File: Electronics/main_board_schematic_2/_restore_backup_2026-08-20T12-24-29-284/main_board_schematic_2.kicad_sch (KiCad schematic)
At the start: 6 parts, among them J1 Conn_01x02_Pin, J2 Conn_01x02_Socket, U1 DEVKIT_V1_ESP32-WROOM-32, U2 L7805

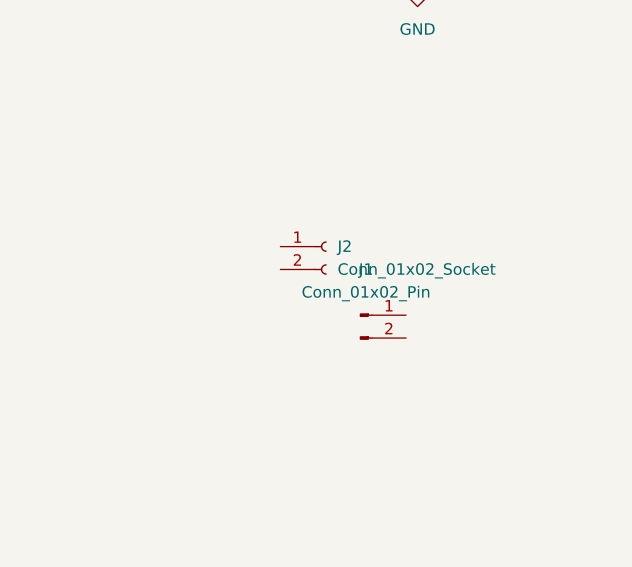
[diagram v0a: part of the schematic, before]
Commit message: start kicad version of board
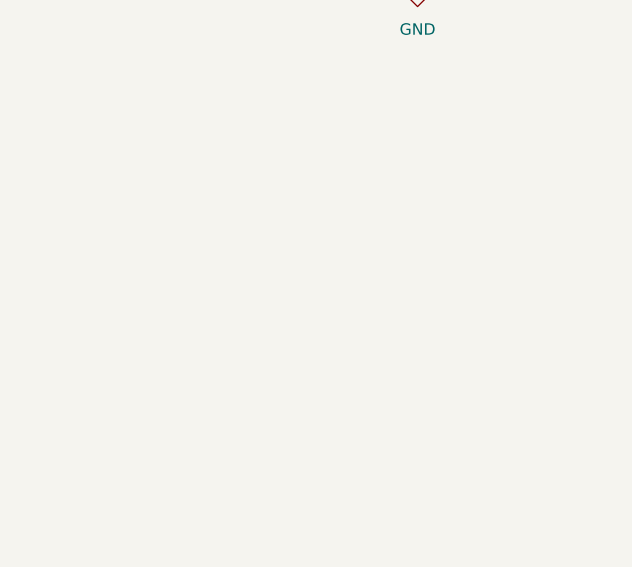
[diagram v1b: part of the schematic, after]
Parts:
- removed J1: Conn_01x02_Pin, Connector_JST:JST_XH_B2B-XH-AM_1x02_P2.50mm_Vertical, symbol Connector:Conn_01x02_Pin
- removed J2: Conn_01x02_Socket, Connector_JST:JST_XH_B2B-XH-A_1x02_P2.50mm_Vertical, symbol Connector:Conn_01x02_Socket
- U2: footprint Package_TO_SOT_THT:TO-220F-3_Horizontal_TabDown -> (none)
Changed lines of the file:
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@@
-	)
-	(symbol
-		(lib_id "Connector:Conn_01x02_Socket")
-		(at 203.2 82.55 0)
-		(unit 1)
-		(body_style 1)
-		(exclude_from_sim no)
-		(in_bom yes)
-		(on_board yes)
-		(in_pos_files yes)
-		(dnp no)
-		(fields_autoplaced yes)
-		(property "Reference" "J2"
-			(at 204.47 82.5499 0)
-			(show_name no)
-			(do_not_autoplace no)
-			(effects
-				(font
-					(size 1.27 1.27)
-				)
-				(justify left)
-			)
-		)
-		(property "Value" "Conn_01x02_Socket"
-			(at 204.47 85.0899 0)
-			(show_name no)
-			(do_not_autoplace no)
-			(effects
-				(font
-					(size 1.27 1.27)
-				)
-				(justify left)
-			)
-		)
-		(property "Footprint" "Connector_JST:JST_XH_B2B-XH-A_1x02_P2.50mm_Vertical"
-			(at 203.2 82.55 0)
-			(hide yes)
-			(show_name no)
-			(do_not_autoplace no)
-			(effects
-				(font
-					(size 1.27 1.27)
-				)
-			)
-		)
-		(property "Datasheet" ""
-			(at 203.2 82.55 0)
-			(hide yes)
-			(show_name no)
-			(do_not_autoplace no)
-			(effects
-				(font
-					(size 1.27 1.27)
-				)
-			)
-		)
-		(property "Description" "Generic connector, single row, 01x02, script generated"
-			(at 203.2 82.55 0)
-			(hide yes)
-			(show_name no)
-			(do_not_autoplace no)
-			(effects
-				(font
-					(size 1.27 1.27)
-				)
-			)
-		)
-		(pin "1"
-		)
-		(pin "2"
-		)
-		(instances
-			(project "main_board_schematic_2"
-				(path "/0f7e1246-28db-45f8-bddc-feff77babbfe"
-					(reference "J2")
-					(unit 1)
-				)
-			)
-		)
 	)
 	(symbol
@@
 			)
 		)
-		(property "Footprint" "Package_TO_SOT_THT:TO-220F-3_Horizontal_TabDown"
+		(property "Footprint" ""
 			(at 213.995 49.53 0)
 			(hide yes)
@@
 					(unit 1)
 				)
-			)
-		)
-	)
-	(symbol
-		(lib_id "Connector:Conn_01x02_Pin")
-		(at 207.01 90.17 0)
-		(unit 1)
-		(body_style 1)
-		(exclude_from_sim no)
-		(in_bom yes)
-		(on_board yes)
-		(in_pos_files yes)
-		(dnp no)
-		(fields_autoplaced yes)
-		(property "Reference" "J1"
-			(at 207.645 85.09 0)
-			(show_name no)
-			(do_not_autoplace no)
-			(effects
-				(font
-					(size 1.27 1.27)
-				)
-			)
-		)
-		(property "Value" "Conn_01x02_Pin"
-			(at 207.645 87.63 0)
-			(show_name no)
-			(do_not_autoplace no)
-			(effects
-				(font
-					(size 1.27 1.27)
-				)
-			)
-		)
-		(property "Footprint" "Connector_JST:JST_XH_B2B-XH-AM_1x02_P2.50mm_Vertical"
-			(at 207.01 90.17 0)
-			(hide yes)
-			(show_name no)
-			(do_not_autoplace no)
-			(effects
-				(font
-					(size 1.27 1.27)
-				)
-			)
-		)
-		(property "Datasheet" ""
-			(at 207.01 90.17 0)
-			(hide yes)
-			(show_name no)
-			(do_not_autoplace no)
-			(effects
-				(font
-					(size 1.27 1.27)
-				)
-			)
-		)
-		(property "Description" "Generic connector, single row, 01x02, script generated"
-			(at 207.01 90.17 0)
-			(hide yes)
-			(show_name no)
-			(do_not_autoplace no)
-			(effects
-				(font
-					(size 1.27 1.27)
-				)
-			)
-		)
-		(pin "1"
-		)
-		(pin "2"
-		)
-		(instances
-			(project "main_board_schematic_2"
-				(path "/0f7e1246-28db-45f8-bddc-feff77babbfe"
-					(reference "J1")
-					(unit 1)
-				)
